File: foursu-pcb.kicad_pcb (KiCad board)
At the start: 2 copper layers, 71.4 x 38.1 mm, 24 parts, among them SW1 SW_Push, U1 ATmega32U4-AU, Y1 16MHz

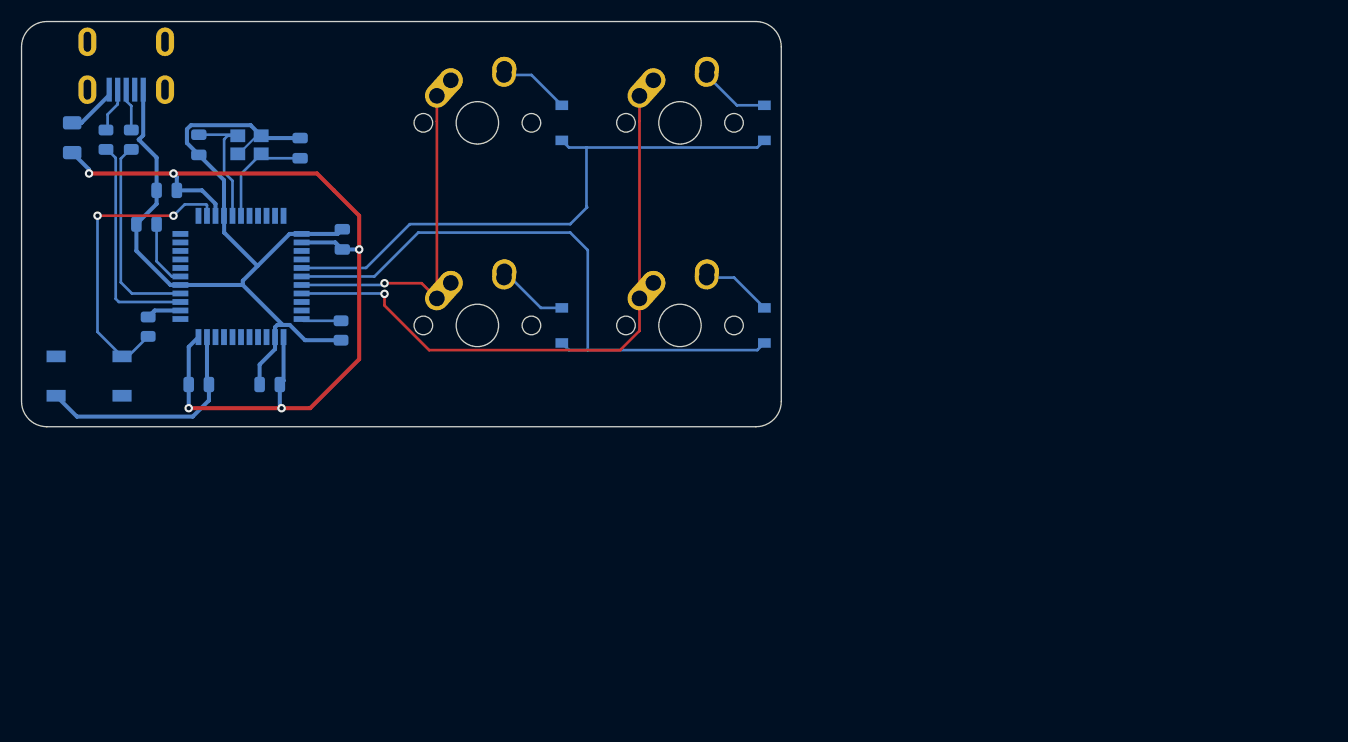
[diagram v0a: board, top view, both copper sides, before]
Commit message: finished first prototype?
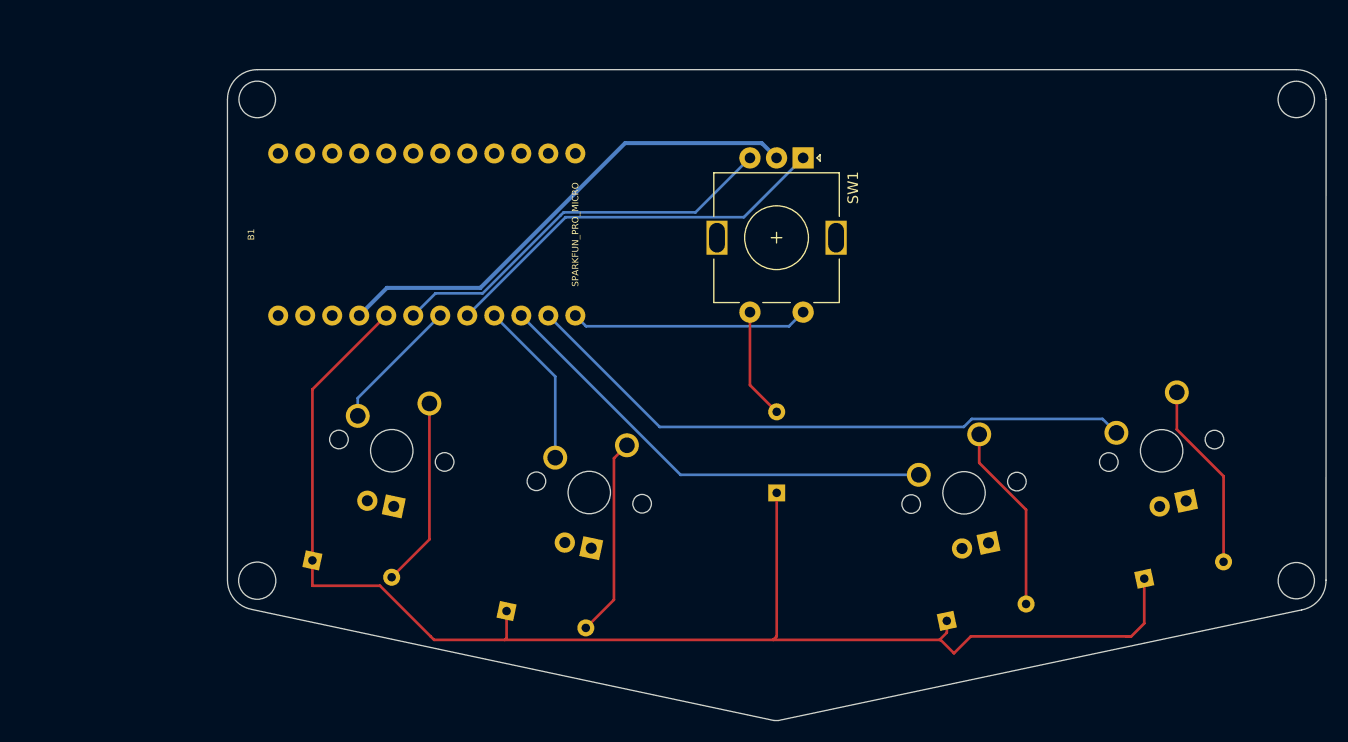
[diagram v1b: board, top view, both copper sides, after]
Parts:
- removed C1, C5, C6: 0.1uF, Capacitor_SMD:C_0805_2012Metric
- removed C2, C3: 22pF, Capacitor_SMD:C_0805_2012Metric
- removed C4: 1uF, Capacitor_SMD:C_0805_2012Metric
- removed C7: 10uF, Capacitor_SMD:C_0805_2012Metric
- removed F1: Polyfuse, Fuse:Fuse_1206_3216Metric
- removed R1, R2: 22, Resistor_SMD:R_0805_2012Metric
- removed R3, R4: 10k, Resistor_SMD:R_0805_2012Metric
- removed U1: ATmega32U4-AU, Package_QFP:TQFP-44_10x10mm_P0.8mm
- removed USB1: Molex-0548190519, random-keyboard-parts:Molex-0548190589
- removed Y1: 16MHz, Crystal:Crystal_SMD_3225-4Pin_3.2x2.5mm
- added B1: SPARKFUN_PRO_MICRO, Boards:SPARKFUN_PRO_MICRO, F.Cu at (57.5, 137.5)
- added D5: 1N4148, Diode_THT:D_DO-35_SOD27_P7.62mm_Horizontal, B.Cu at (91.6, 161.8)
- D1, D2, D3, D4: value SOD-123 -> 1N4148; footprint Diode_SMD:D_SOD-123 -> Diode_THT:D_DO-35_SOD27_P7.62mm_Horizontal
- MX1, MX2, MX3, MX4: value MX-NoLED -> MX-LED; footprint MX_Alps_Hybrid:MX-1U-NoLED -> MX_Only:MXOnly-1U
- SW1: value SW_Push -> Rotary_Encoder_Switch; footprint random-keyboard-parts:SKQG-1155865 -> Rotary_Encoder:RotaryEncoder_Alps_EC11E-Switch_Vertical_H20mm; moved to F.Cu
- moved SW1 70.2 mm to (94.1, 130.3), turned to 270 degrees
- moved D3 49.9 mm to (107.6, 173.8), turned to 12 degrees
- moved D1 47.4 mm to (48.0, 168.1), turned to 348 degrees
- moved MX4 46.8 mm to (127.8, 157.8), turned to 12 degrees
- moved MX3 43.9 mm to (109.3, 161.8), turned to 12 degrees
- moved D4 42.9 mm to (126.2, 169.9), turned to 12 degrees
- moved MX1 31.9 mm to (55.5, 157.8), turned to 348 degrees
- moved D2 27.4 mm to (66.2, 172.9), turned to 348 degrees
- moved MX2 18.9 mm to (74.0, 161.8), turned to 348 degrees
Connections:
- D2 pad 1: ROW1 -> ROW0
- D4 pad 1: ROW1 -> ROW0
- MX2 pad 1: COL0 -> COL1
- MX3 pad 1: COL1 -> COL2
- MX4 pad 1: COL1 -> COL3
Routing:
- net +5V: track 91.0 -> 0.00 mm, vias 5 -> 0
- net ROW0: track 54.5 -> 133.6 mm
- net GND: track 110.4 -> 46.5 mm
- net COL3: track 0.00 -> 58.6 mm
- net ROW1: track 58.3 -> 0.00 mm
- net COL2: track 0.00 -> 43.6 mm
- net COL1: track 57.5 -> 15.7 mm, vias 1 -> 0
- net ENC0: track 0.00 -> 37.8 mm
- net ENC1: track 0.00 -> 37.7 mm
- net Net-(R3-Pad2): track 29.2 -> 0.00 mm, vias 2 -> 0
- net COL4: track 0.00 -> 22.4 mm
- net Net-(R1-Pad1): track 20.7 -> 0.00 mm
- net COL0: track 32.4 -> 12.6 mm, vias 1 -> 0
- net Net-(R2-Pad1): track 19.0 -> 0.00 mm
- net Net-(C3-Pad1): track 12.7 -> 0.00 mm
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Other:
- board size 71.4 x 38.1 mm -> 103.3 x 61.2 mm
